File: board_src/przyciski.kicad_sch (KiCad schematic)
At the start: 9 parts, among them J5 Conn_01x08

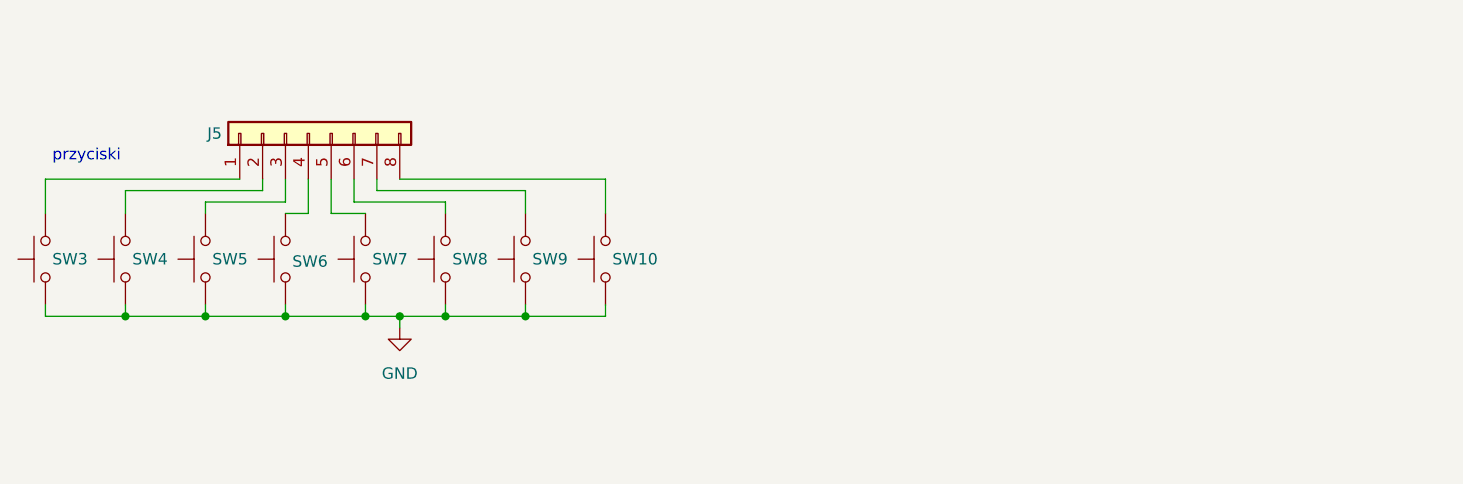
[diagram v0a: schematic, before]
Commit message: wersja 3d
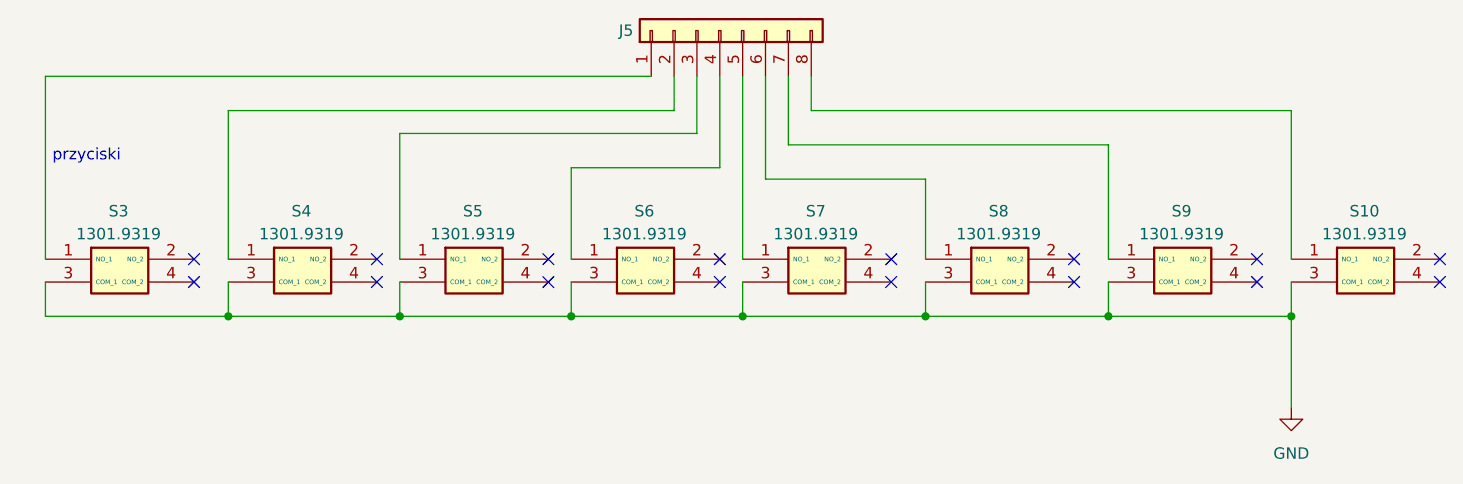
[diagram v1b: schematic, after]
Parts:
- removed SW10, SW3, SW4, SW5, SW6, SW7, SW8, SW9: ~, Button_Switch_THT:SW_PUSH_6mm, symbol Switch:SW_Push
- added S10, S3, S4, S5, S6, S7, S8, S9: 1301.9319, footprints:przycisk, symbol przycisk:1301.9319
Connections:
- net GND: now also S10.3 (COM_1), S3.3 (COM_1), S4.3 (COM_1), S5.3 (COM_1), S6.3 (COM_1), S7.3 (COM_1), S8.3 (COM_1), S9.3 (COM_1)
- net at J5.1 (Pin_1): now also S3.1 (NO_1)
- net at J5.2 (Pin_2): now also S4.1 (NO_1)
- net at J5.3 (Pin_3): now also S5.1 (NO_1)
- net at J5.4 (Pin_4): now also S6.1 (NO_1)
- net at J5.5 (Pin_5): now also S7.1 (NO_1)
- net at J5.6 (Pin_6): now also S8.1 (NO_1)
- net at J5.7 (Pin_7): now also S9.1 (NO_1)
- net at J5.8 (Pin_8): now also S10.1 (NO_1)
- no-connect marks 0 -> 16
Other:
- moved on the sheet: J5
